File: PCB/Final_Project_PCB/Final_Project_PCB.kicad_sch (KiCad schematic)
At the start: 35 parts

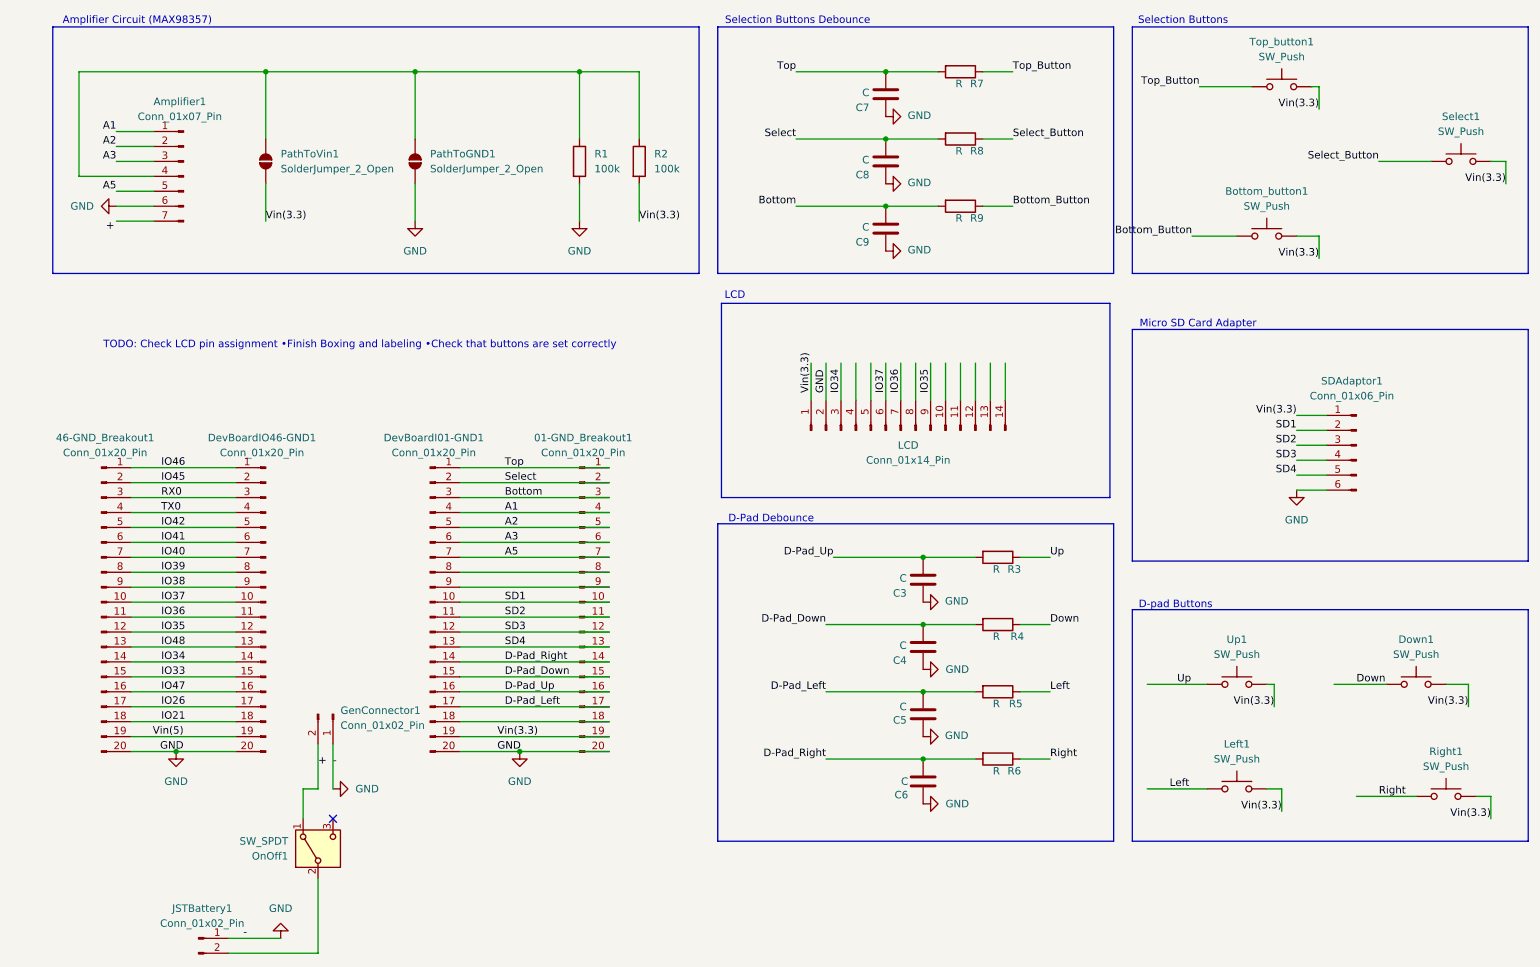
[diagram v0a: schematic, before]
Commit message: updates againnnn
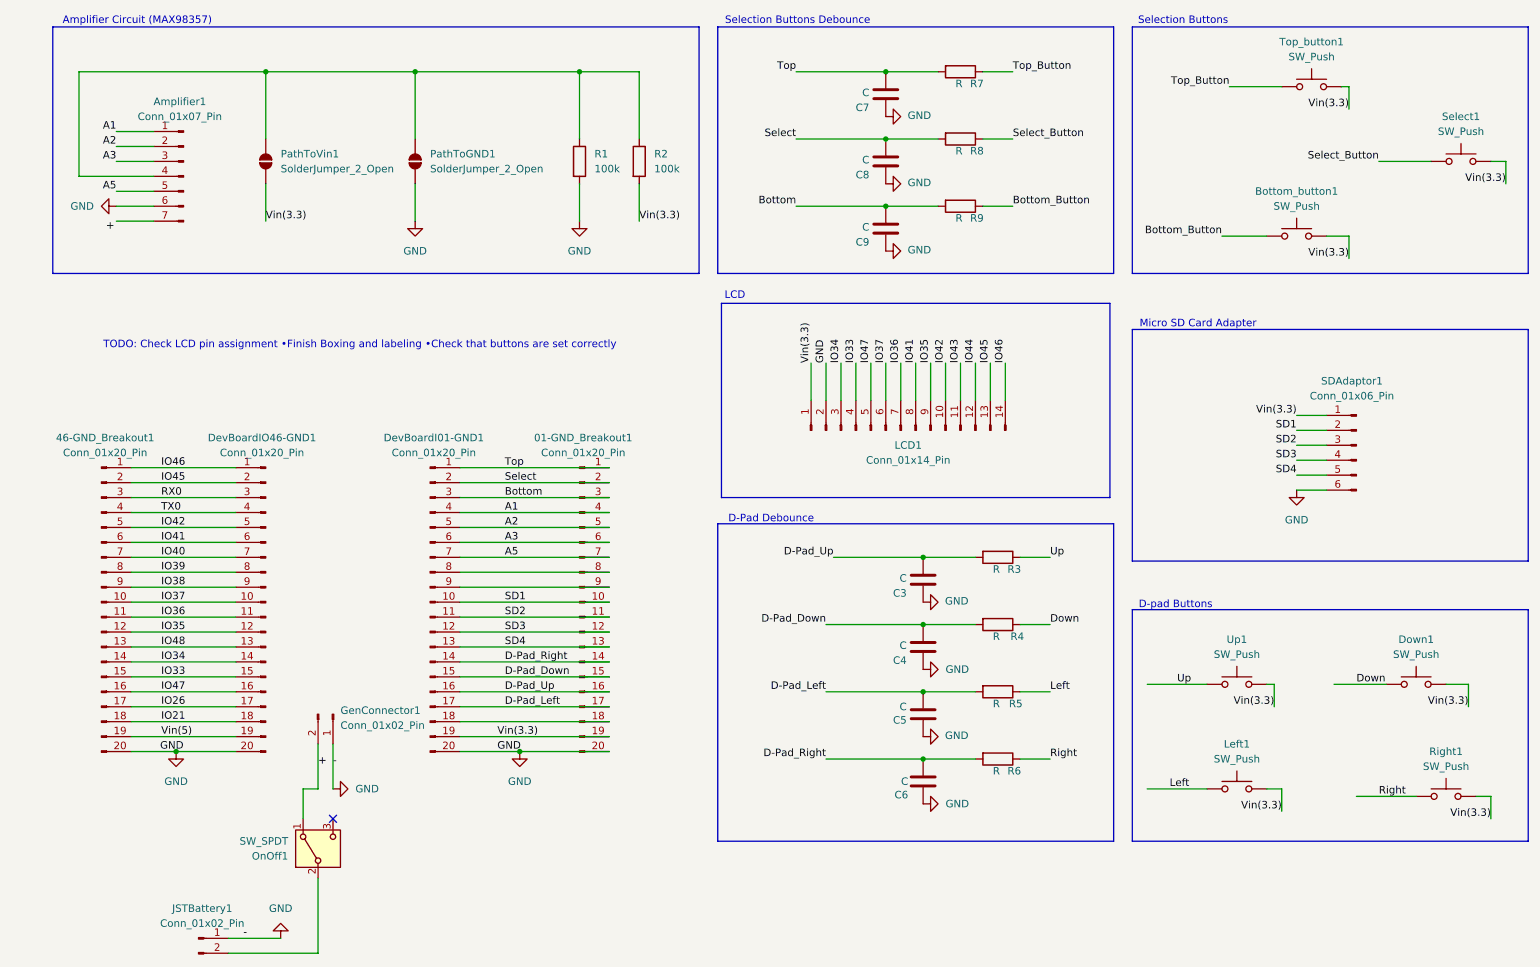
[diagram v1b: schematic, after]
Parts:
- LCD1: renamed from LCD; footprint (none) -> Connector_PinHeader_2.54mm:PinHeader_1x14_P2.54mm_Vertical
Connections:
- net IO33: now also LCD1.4 (Pin_4)
- net IO41: now also LCD1.8 (Pin_8)
- net IO42: now also LCD1.10 (Pin_10)
- net IO45: now also LCD1.13 (Pin_13)
- net IO46: now also LCD1.14 (Pin_14)
- net IO47: now also LCD1.5 (Pin_5)
- net IO43: now reaches LCD1.11 (Pin_11)
- net IO44: now reaches LCD1.12 (Pin_12)
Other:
- moved on the sheet: Bottom_button1, Top_button1
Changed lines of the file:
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@@
 	(wire
 		(pts
-			(xy 180.34 76.2) (xy 180.34 82.55)
+			(xy 157.48 76.2) (xy 157.48 82.55)
 		)
 		(stroke
@@
 	(wire
 		(pts
-			(xy 157.48 76.2) (xy 157.48 82.55)
+			(xy 180.34 76.2) (xy 180.34 82.55)
 		)
 		(stroke
@@
 	(wire
 		(pts
+			(xy 170.18 76.2) (xy 170.18 82.55)
+		)
+		(stroke
+			(width 0)
+			(type default)
+		)
+	)
+	(wire
+		(pts
 			(xy 64.77 26.67) (xy 64.77 38.1)
 		)
@@
 	(wire
 		(pts
-			(xy 160.02 76.2) (xy 160.02 82.55)
-		)
-		(stroke
-			(width 0)
-			(type default)
-		)
-	)
-	(wire
-		(pts
 			(xy 41.91 111.76) (xy 59.69 111.76)
 		)
@@
 	(wire
 		(pts
-			(xy 170.18 76.2) (xy 170.18 82.55)
-		)
-		(stroke
-			(width 0)
-			(type default)
-		)
-	)
-	(wire
-		(pts
 			(xy 97.79 134.62) (xy 123.19 134.62)
 		)
@@
 	(wire
 		(pts
-			(xy 222.25 54.61) (xy 229.87 54.61)
+			(xy 227.33 54.61) (xy 234.95 54.61)
 		)
 		(stroke
@@
 	(wire
 		(pts
-			(xy 162.56 76.2) (xy 162.56 82.55)
+			(xy 154.94 49.53) (xy 170.18 49.53)
 		)
 		(stroke
@@
 	(wire
 		(pts
-			(xy 154.94 49.53) (xy 170.18 49.53)
+			(xy 97.79 109.22) (xy 123.19 109.22)
 		)
 		(stroke
@@
 	(wire
 		(pts
-			(xy 97.79 109.22) (xy 123.19 109.22)
+			(xy 162.56 76.2) (xy 162.56 82.55)
 		)
 		(stroke
@@
 	(wire
 		(pts
+			(xy 160.02 76.2) (xy 160.02 82.55)
+		)
+		(stroke
+			(width 0)
+			(type default)
+		)
+	)
+	(wire
+		(pts
 			(xy 214.63 148.59) (xy 224.79 148.59)
 		)
@@
 	(wire
 		(pts
-			(xy 223.52 29.21) (xy 232.41 29.21)
+			(xy 228.6 29.21) (xy 237.49 29.21)
 		)
 		(stroke
@@
 	(wire
 		(pts
-			(xy 243.84 54.61) (xy 243.84 58.42)
+			(xy 248.92 54.61) (xy 248.92 58.42)
 		)
 		(stroke
@@
 	(wire
 		(pts
-			(xy 242.57 29.21) (xy 243.84 29.21)
+			(xy 247.65 29.21) (xy 248.92 29.21)
 		)
 		(stroke
@@
 	(wire
 		(pts
-			(xy 243.84 29.21) (xy 243.84 33.02)
+			(xy 248.92 29.21) (xy 248.92 33.02)
 		)
 		(stroke
@@
 	(wire
 		(pts
-			(xy 240.03 54.61) (xy 243.84 54.61)
+			(xy 245.11 54.61) (xy 248.92 54.61)
 		)
 		(stroke
@@
 	)
 	(label "IO37"
-		(at 170.18 81.28 90)
+		(at 170.18 76.2 90)
 		(fields_autoplaced yes)
 		(effects
@@
 		)
 	)
+	(label "IO47"
+		(at 167.64 76.2 90)
+		(fields_autoplaced yes)
+		(effects
+			(font
+				(size 1.27 1.27)
+			)
+			(justify left bottom)
+		)
+	)
 	(label "D-Pad_Left"
 		(at 160.02 132.08 180)
@@
 	)
 	(label "GND"
-		(at 160.02 81.28 90)
+		(at 160.02 76.2 90)
 		(fields_autoplaced yes)
 		(effects
@@
 		)
 	)
+	(label "IO33"
+		(at 165.1 76.2 90)
+		(fields_autoplaced yes)
+		(effects
+			(font
+				(size 1.27 1.27)
+			)
+			(justify left bottom)
+		)
+	)
 	(label "SD4"
 		(at 105.41 124.46 0)
@@
 	)
 	(label "Bottom_Button"
-		(at 222.25 54.61 180)
+		(at 227.33 54.61 180)
 		(fields_autoplaced yes)
 		(effects
@@
 		)
 	)
+	(label "IO46"
+		(at 190.5 76.2 90)
+		(fields_autoplaced yes)
+		(effects
+			(font
+				(size 1.27 1.27)
+			)
+			(justify left bottom)
+		)
+	)
 	(label "Vin(3.3)"
 		(at 64.77 52.07 0)
@@
 	)
 	(label "Top_Button"
-		(at 223.52 29.21 180)
+		(at 228.6 29.21 180)
 		(fields_autoplaced yes)
 		(effects
@@
 	)
 	(label "IO36"
-		(at 172.72 81.28 90)
+		(at 172.72 76.2 90)
 		(fields_autoplaced yes)
 		(effects
@@
 		)
 	)
+	(label "IO43"
+		(at 182.88 76.2 90)
+		(fields_autoplaced yes)
+		(effects
+			(font
+				(size 1.27 1.27)
+			)
+			(justify left bottom)
+		)
+	)
 	(label "Up"
 		(at 198.12 109.22 0)
@@
 		)
 	)
+	(label "IO42"
+		(at 180.34 76.2 90)
+		(fields_autoplaced yes)
+		(effects
+			(font
+				(size 1.27 1.27)
+			)
+			(justify left bottom)
+		)
+	)
 	(label "IO35"
 		(at 46.99 121.92 0)
@@
 	)
 	(label "Vin(3.3)"
-		(at 157.48 81.28 90)
+		(at 157.48 76.2 90)
 		(fields_autoplaced yes)
 		(effects
@@
 	)
 	(label "Vin(5)"
-		(at 50.8 139.7 180)
+		(at 46.99 139.7 0)
 		(fields_autoplaced yes)
 		(effects
@@
 				(size 1.27 1.27)
 			)
-			(justify right bottom)
+			(justify left bottom)
 		)
 	)
 	(label "Vin(3.3)"
-		(at 243.84 58.42 180)
+		(at 248.92 58.42 180)
 		(fields_autoplaced yes)
 		(effects
@@
 	)
 	(label "IO35"
-		(at 177.8 81.28 90)
+		(at 177.8 76.2 90)
 		(fields_autoplaced yes)
 		(effects
@@
 		)
 	)
+	(label "IO41"
+		(at 175.26 76.2 90)
+		(fields_autoplaced yes)
+		(effects
+			(font
+				(size 1.27 1.27)
+			)
+			(justify left bottom)
+		)
+	)
 	(label "Select_Button"
 		(at 254 41.91 180)
@@
 	)
 	(label "IO34"
-		(at 162.56 81.28 90)
+		(at 162.56 76.2 90)
 		(fields_autoplaced yes)
 		(effects
@@
 		)
 	)
+	(label "IO44"
+		(at 185.42 76.2 90)
+		(fields_autoplaced yes)
+		(effects
+			(font
+				(size 1.27 1.27)
+			)
+			(justify left bottom)
+		)
+	)
 	(label "IO45"
 		(at 46.99 96.52 0)
@@
 		)
 	)
+	(label "IO45"
+		(at 187.96 76.2 90)
+		(fields_autoplaced yes)
+		(effects
+			(font
+				(size 1.27 1.27)
+			)
+			(justify left bottom)
+		)
+	)
 	(label "Vin(3.3)"
 		(at 240.03 85.09 180)
@@
 	)
 	(label "Vin(3.3)"
-		(at 243.84 33.02 180)
+		(at 248.92 33.02 180)
 		(fields_autoplaced yes)
 		(effects
@@
 	(symbol
 		(lib_id "Switch:SW_Push")
-		(at 234.95 54.61 0)
+		(at 240.03 54.61 0)
 		(unit 1)
 		(exclude_from_sim no)
@@
 		(fields_autoplaced yes)
 		(property "Reference" "Bottom_button1"
-			(at 234.95 46.99 0)
+			(at 240.03 46.99 0)
 			(effects
 				(font
@@
 		)
 		(property "Value" "SW_Push"
-			(at 234.95 49.53 0)
+			(at 240.03 49.53 0)
 			(effects
 				(font
@@
 		)
 		(property "Footprint" "Button_Switch_SMD:SW_SPST_PTS810"
-			(at 234.95 49.53 0)
+			(at 240.03 49.53 0)
 			(effects
 				(font
@@
 		)
 		(property "Datasheet" "~"
-			(at 234.95 49.53 0)
+			(at 240.03 49.53 0)
 			(effects
 				(font
@@
 		)
 		(property "Description" "Push button switch, generic, two pins"
-			(at 234.95 54.61 0)
+			(at 240.03 54.61 0)
 			(effects
 				(font
@@
 		(dnp no)
 		(fields_autoplaced yes)
-		(property "Reference" "LCD"
+		(property "Reference" "LCD1"
 			(at 173.99 90.17 90)
 			(effects
@@
 			)
 		)
-		(property "Footprint" ""
+		(property "Footprint" "Connector_PinHeader_2.54mm:PinHeader_1x14_P2.54mm_Vertical"
 			(at 172.72 87.63 0)
 			(effects
@@
 			(project ""
 				(path "/539b41c1-4420-4cfd-92b7-a29c74941d81"
-					(reference "LCD")
+					(reference "LCD1")
 					(unit 1)
 				)
@@
 	(symbol
 		(lib_id "Switch:SW_Push")
-		(at 237.49 29.21 0)
+		(at 242.57 29.21 0)
 		(unit 1)
 		(exclude_from_sim no)
@@
 		(fields_autoplaced yes)
 		(property "Reference" "Top_button1"
-			(at 237.49 21.59 0)
+			(at 242.57 21.59 0)
 			(effects
 				(font
@@
 		)
 		(property "Value" "SW_Push"
-			(at 237.49 24.13 0)
+			(at 242.57 24.13 0)
 			(effects
 				(font
@@
 		)
 		(property "Footprint" "Button_Switch_SMD:SW_SPST_PTS810"
-			(at 237.49 24.13 0)
+			(at 242.57 24.13 0)
 			(effects
 				(font
@@
 		)
 		(property "Datasheet" "~"
-			(at 237.49 24.13 0)
+			(at 242.57 24.13 0)
 			(effects
 				(font
@@
 		)
 		(property "Description" "Push button switch, generic, two pins"
-			(at 237.49 29.21 0)
+			(at 242.57 29.21 0)
 			(effects
 				(font
